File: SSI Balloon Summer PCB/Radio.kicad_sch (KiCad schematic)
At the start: 6 parts, among them J3 Conn_Coaxial, U1 RFM95W-915S2, U5 DRA818V

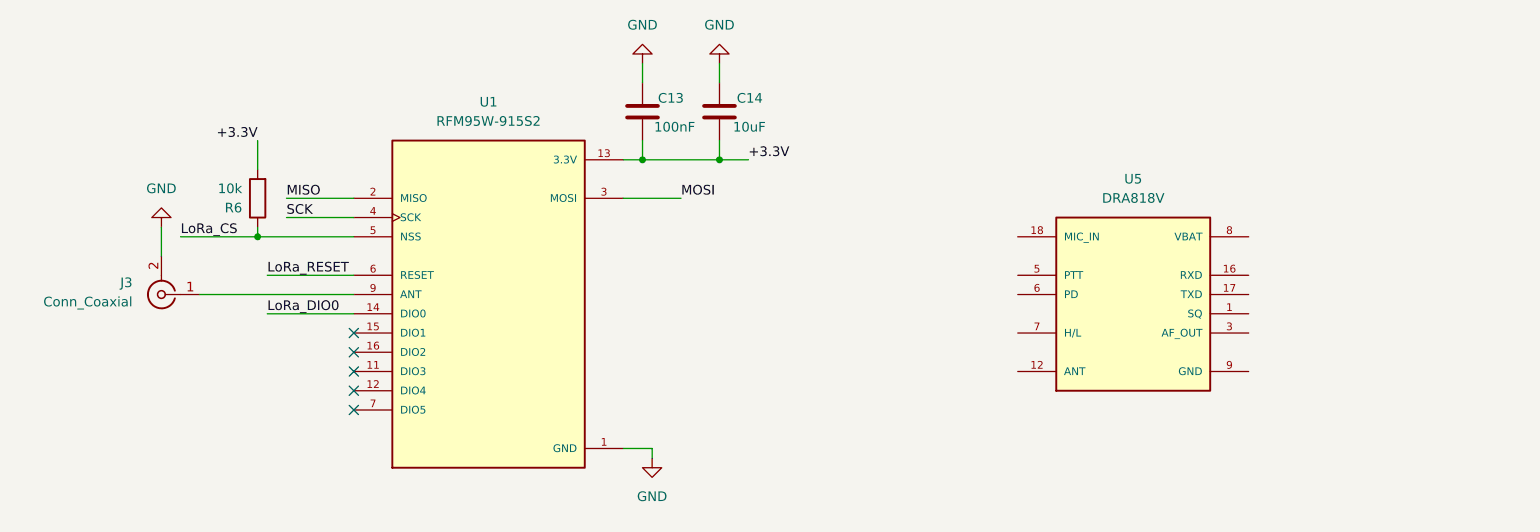
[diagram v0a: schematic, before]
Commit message: APRS work - MIC_IN pin left
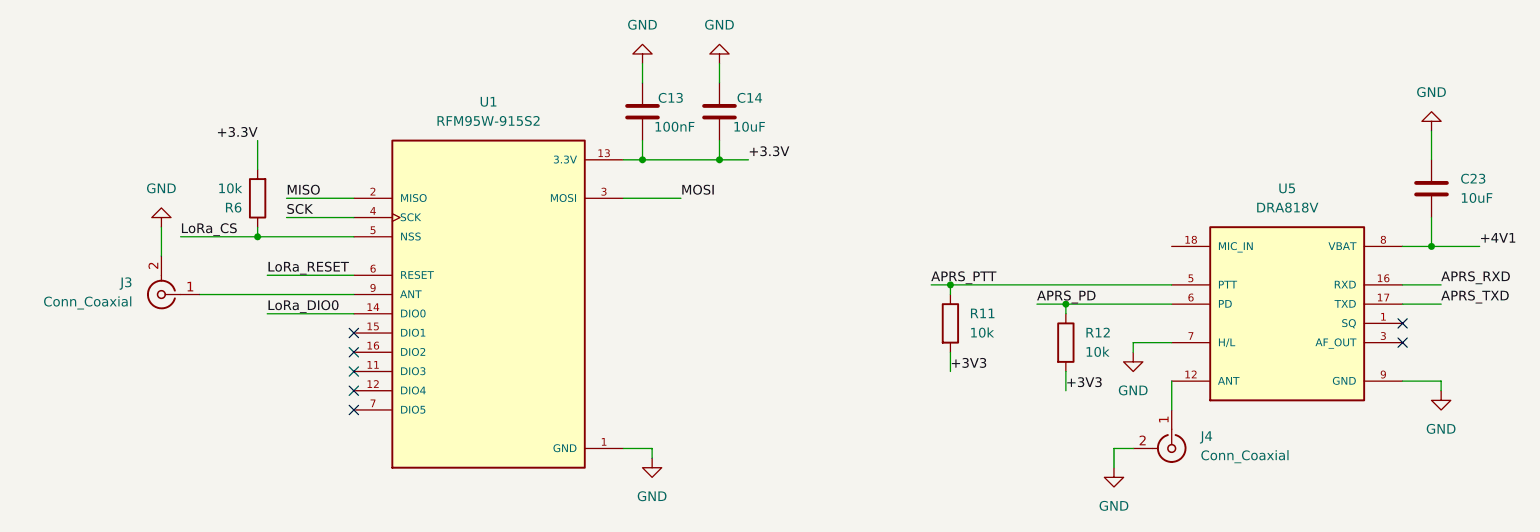
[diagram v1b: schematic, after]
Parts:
- added C23: 10uF, symbol Device:C
- added J4: Conn_Coaxial, symbol Connector:Conn_Coaxial
- added R11, R12: 10k, symbol Device:R
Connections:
- net GND: now also U5.7 (H/L), C23.1, J4.2 (Ext)
- net at U5.12 (ANT): now also J4.1 (In)
- net APRS_RXD: now reaches U5.16 (RXD)
- net APRS_TXD: now reaches U5.17 (TXD)
- net APRS_PTT: now reaches U5.5 (PTT)
- net APRS_PTT: now also R11.1
- net APRS_PD: now reaches U5.6 (PD)
- net APRS_PD: now also R12.1
- net +4V1: now reaches U5.8 (VBAT)
- net +4V1: now also C23.2
- new net +3V3: R11.2, R12.2
- no-connect marks 5 -> 7
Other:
- moved on the sheet: U5
